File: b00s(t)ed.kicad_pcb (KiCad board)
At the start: 2 copper layers, 3 parts, among them P1 XT60PW, P2 XT60PW, Q1 IRL7472L1

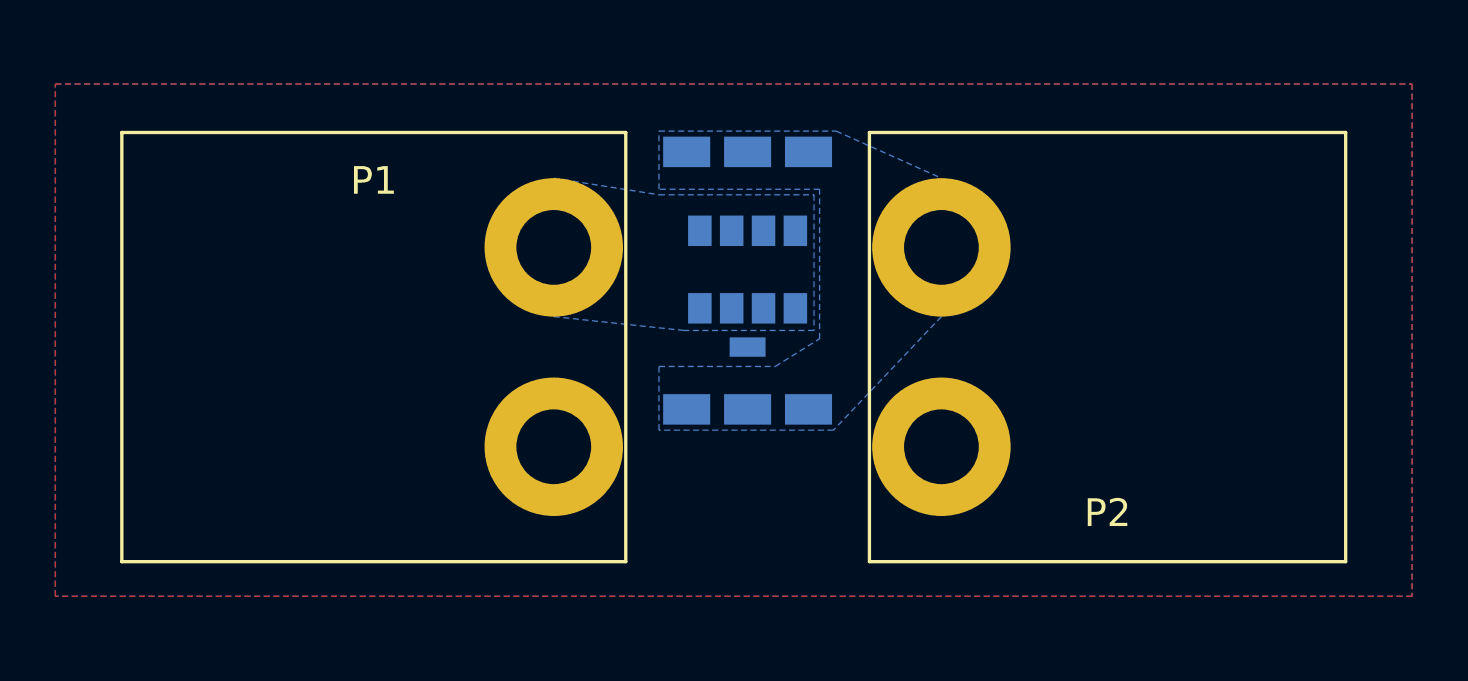
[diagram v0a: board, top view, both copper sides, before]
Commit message: backup
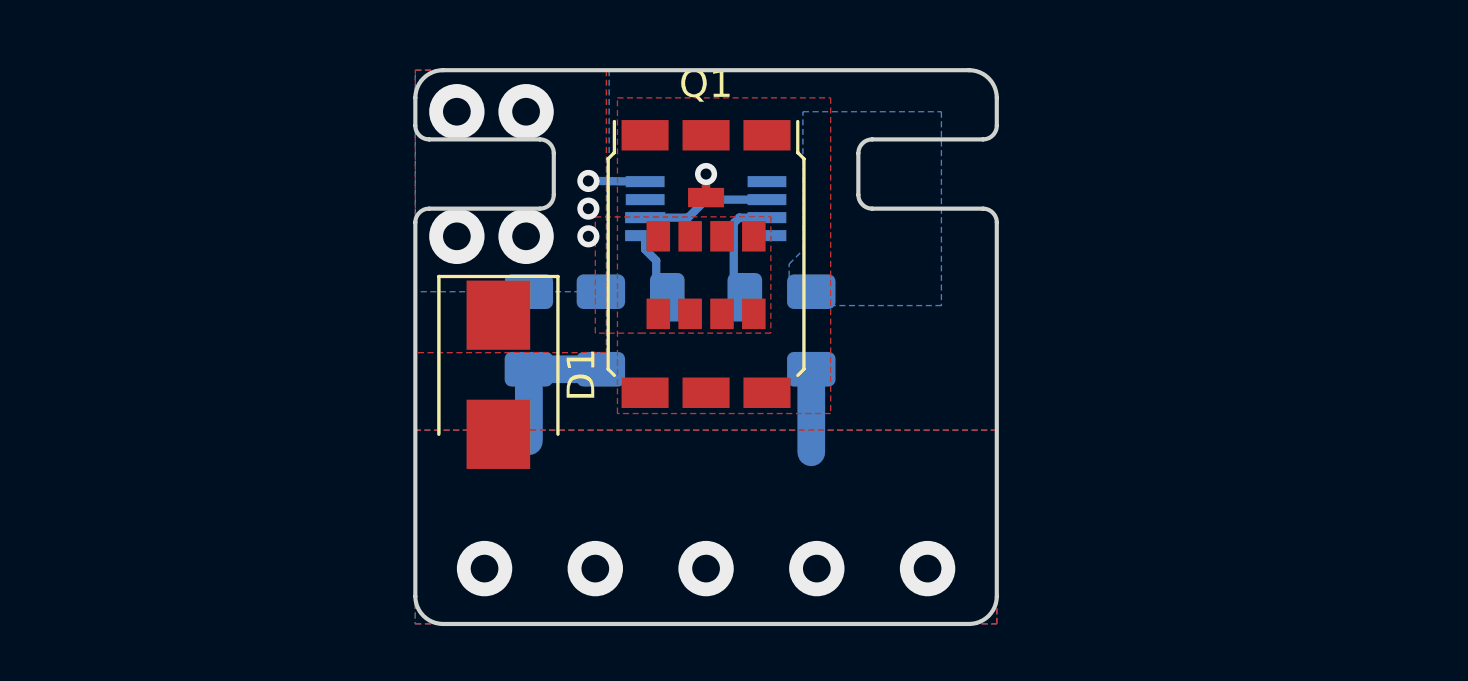
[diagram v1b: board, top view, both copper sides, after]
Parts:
- removed P1: XT60PW, Connector:XT60PW-M
- removed P2: XT60PW, Connector:XT60PW-F
- added C1: C, Capacitor_SMD:C_1206_3216Metric, B.Cu at (133.6, 69.4)
- added C2: C, Capacitor_SMD:C_1206_3216Metric, B.Cu at (136.2, 69.4)
- added C3: C, Capacitor_SMD:C_1206_3216Metric, B.Cu at (140.0, 68.2)
- added C4: C, Capacitor_SMD:C_1206_3216Metric, B.Cu at (143.8, 69.4)
- added D1: D, Diode_SMD:D_SMB, F.Cu at (132.5, 71.0)
- added U1: LM74610-Q1, Package_SO:S-PDSO-G8, B.Cu at (140.0, 65.0)
- Q1: moved to F.Cu
- moved Q1 1.62 mm to (140.0, 67.0), turned to 270 degrees
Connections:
- Q1 pad 1: Net-(P2-Pad+) -> /OUT
- Q1 pad 2: (no net) -> Net-(Q1-Pad2)
- Q1 pad 3: Net-(P1-Pad+) -> +BATT
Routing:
- net -BATT: track 0.00 -> 8.20 mm, vias 0 -> 5
- net Net-(Q1-Pad2): track 0.00 -> 6.44 mm, vias 0 -> 1
- net Net-(C3-Pad2): track 0.00 -> 4.12 mm
- net Net-(C3-Pad1): track 0.00 -> 2.56 mm
- net +BATT: track 0.00 -> 1.80 mm, vias 0 -> 7
- added copper zone on B.Cu, net +BATT
- added copper zone on F.Cu, net +BATT
- added copper zone on B.Cu, net -BATT
- added copper zone on F.Cu, net -BATT
- added copper zone on B.Cu, net /OUT
- added copper zone on F.Cu, net /OUT
- removed copper zone on B.Cu, net GND
- removed copper zone on F.Cu, net GND
- removed copper zone on B.Cu, net Net-(P1-Pad+)
- removed copper zone on B.Cu, net Net-(P2-Pad+)
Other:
- board outline added: 21 x 20 mm
- net class Default: trace_width 0.15 -> 0.3
- net class HV removed

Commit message: First version ready for order
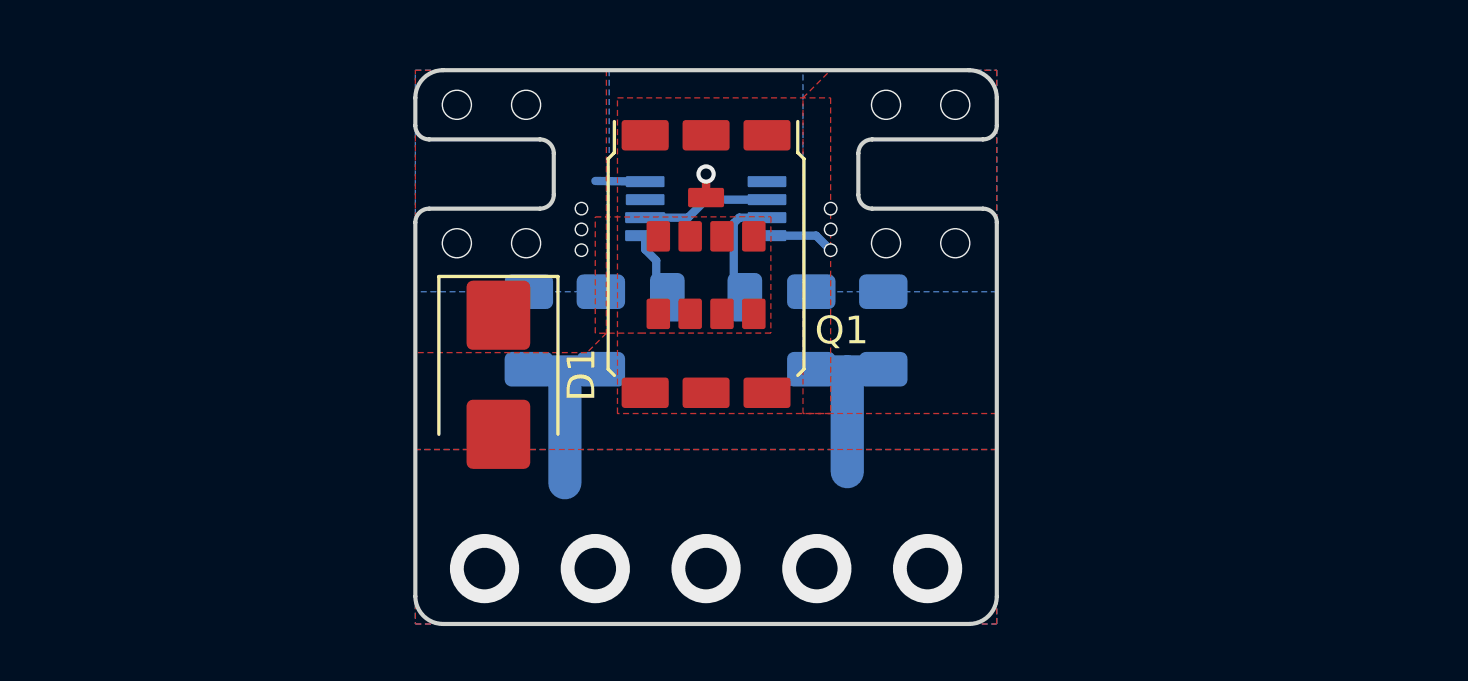
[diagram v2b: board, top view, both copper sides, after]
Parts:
- added C5: C, Capacitor_SMD:C_1206_3216Metric, B.Cu at (146.4, 69.4)
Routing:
- net -BATT: track 8.20 -> 12.5 mm
- net /OUT: track 0.00 -> 2.52 mm, vias 0 -> 7
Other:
- net class Default: via_dia 0.8 -> 0.7
- rule pad_to_mask_clearance: 0.051 -> 0
- rule solder_mask_min_width: 0.25 -> 0.2
- board text added: "2019-02-02"
- board text added: "b00s(t)ed"
- board text added: "by turbo function"

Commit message: ordered
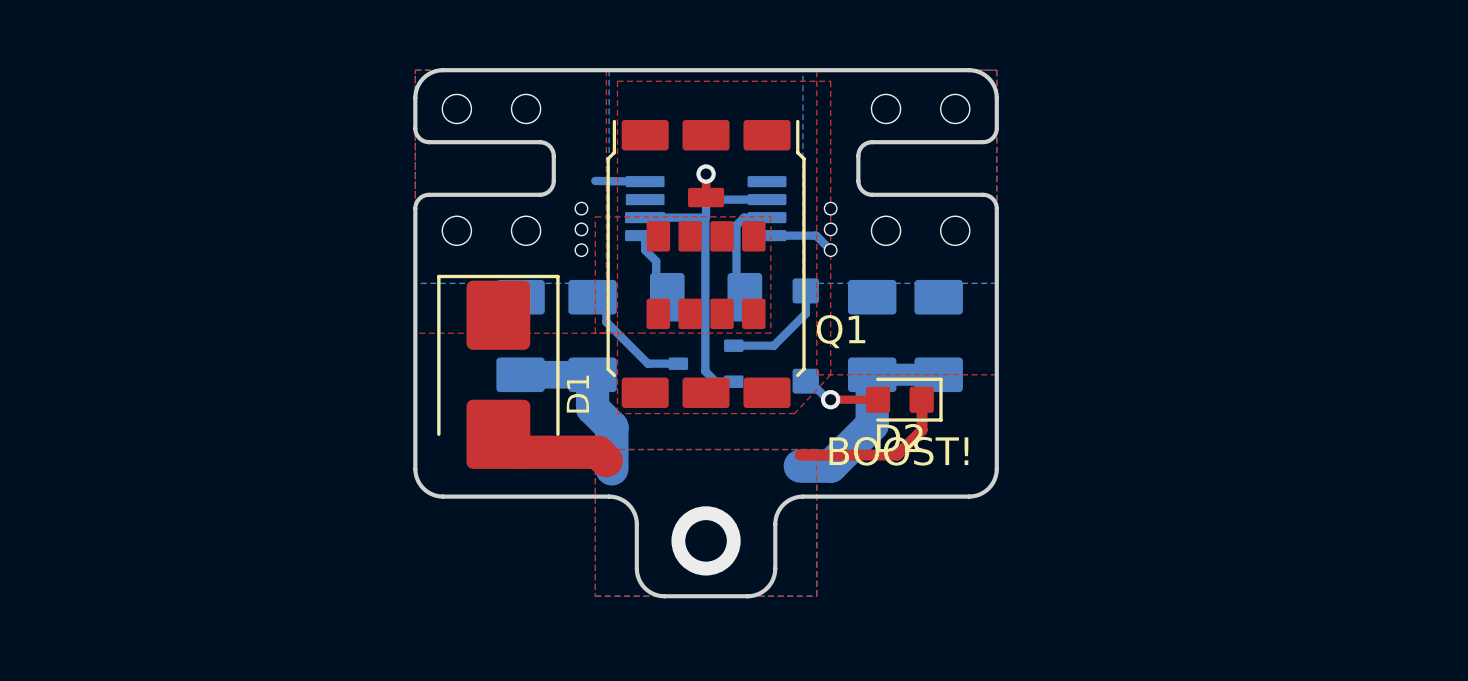
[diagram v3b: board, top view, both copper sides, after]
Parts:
- added D2: VLMTG1400, Diode_SMD:D_0603_1608Metric, F.Cu at (147.0, 71.9)
- added Q2: 2N7002W, Package_TO_SOT_SMD:SOT-323_SC-70, B.Cu at (140.0, 70.6)
- added U2: NSI50010YT1G, Digikey:SOD-123, B.Cu at (143.6, 69.6)
- Q1: value IRL7472L1 -> IRF7739L1
- moved C4 2.21 mm to (146.0, 69.6)
- moved C5 2.01 mm to (148.4, 69.6)
- moved C1 0.36 mm to (133.3, 69.6)
- moved C2 0.36 mm to (135.9, 69.6)
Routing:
- net -BATT: track 12.5 -> 23.8 mm, vias 5 -> 1
- net Net-(Q1-Pad2): track 6.44 -> 13.5 mm
- net +BATT: track 1.80 -> 6.13 mm
- net Net-(Q2-Pad1): track 0.00 -> 3.88 mm
- net Net-(D2-Pad2): track 0.00 -> 3.01 mm, vias 0 -> 1
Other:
- board size 21 x 20 mm -> 21 x 19 mm
- net class HV added: clearance 0.3, trace_width 0.3, via_dia 0.7, via_drill 0.4
- net class Power added: clearance 0.15, trace_width 1.2, via_dia 0.7, via_drill 0.4
- rule pad_to_mask_clearance: 0 -> 0.03
- rule solder_mask_min_width: 0.2 -> 0.15
- board text added: "1-6s"
- board text added: "2019-02-04"
- board text added: "BOOST!"
- board text added: "TURBOfunction.com"
- board text removed: "2019-02-02"
- board text removed: "by turbo function"
